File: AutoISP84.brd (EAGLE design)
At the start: 13 x 34.3 mm, 4 parts, among them J1 MCU, J2 BOARD, U1 ATTINY84-20PU, U2 ATTINY84-20PU

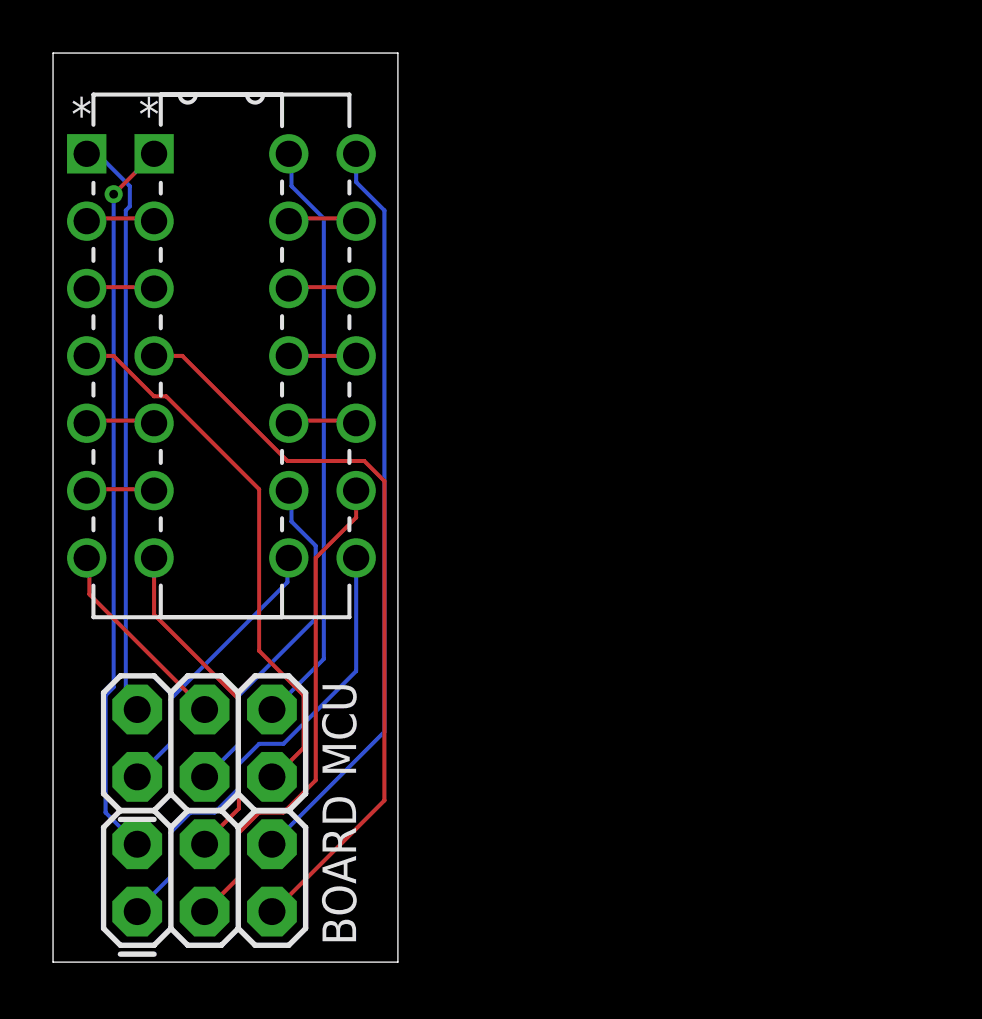
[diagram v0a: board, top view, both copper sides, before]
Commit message: Revise boards for better labelling and sane orientation, add AutoISP328
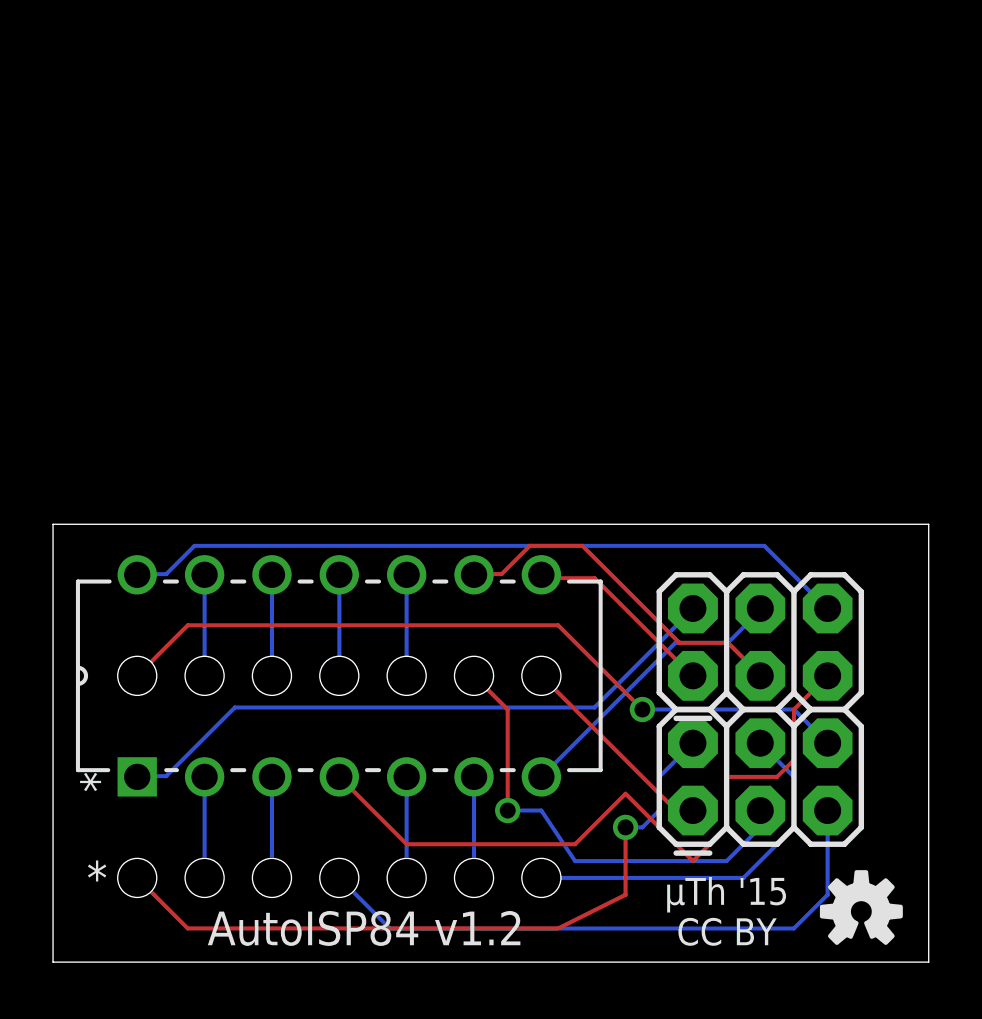
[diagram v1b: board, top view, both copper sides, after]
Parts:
- removed U2: ATTINY84-20PU, Atmel_By_element14_Batch_1-00:DIP254P762X533-14
- added JP1, JP2: (no value), SparkFun-Connectors:1X07_HOLES_ONLY
- added U$1: (no value), SparkFun-Aesthetics:OSHW-LOGO-S
- moved J1 21.3 mm to (24.1, 10.8)
- moved J2 21.3 mm to (24.1, 5.71)
- moved U1 9.55 mm to (18.4, 14.6), turned to 90 degrees
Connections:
- removed net N$11: J2.1, U2.8
- removed net N$13: J2.3, U2.9
- removed net N$9: J2.4, U2.7
- new net N$19: J2.4, JP1.7
- new net N$22: J2.1, JP2.1
- new net N$23: J2.3, JP2.2
- net N$12: now also JP2.6; no longer U2.13
- net N$14: now also JP1.5; no longer U2.5
- net N$15: now also JP1.3; no longer U2.3
- net N$16: now also JP1.2; no longer U2.2
- net N$17: now also JP1.6; no longer U2.6
- net N$18: now also JP2.5; no longer U2.12
- net N$2: now also JP1.1; no longer U2.1
- net N$20: now also JP2.4; no longer U2.11
- net N$21: now also JP2.3; no longer U2.10
- net N$3: now also JP2.7; no longer U2.14
- net N$7: now also JP1.4; no longer U2.4
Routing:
- net N$13: track 18.8 -> 0.00 mm
- net N$11: track 17.8 -> 0.00 mm
- net N$23: track 0.00 -> 17.3 mm, vias 0 -> 1
- net N$19: track 0.00 -> 14.0 mm
- net N$9: track 12.6 -> 0.00 mm
- net N$22: track 0.00 -> 7.82 mm
- net N$5: track 20.7 -> 26.4 mm
- net N$7: track 28.7 -> 22.9 mm
- net N$4: track 22.4 -> 27.5 mm
- net N$8: track 7.62 -> 10.9 mm
- net N$10: track 10.7 -> 7.34 mm
- net N$1: track 22.1 -> 23.6 mm
- net N$20: track 2.54 -> 3.81 mm
- net N$17: track 2.60 -> 3.81 mm
- net N$18: track 2.60 -> 3.81 mm
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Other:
- board size 13 x 34.3 mm -> 33 x 16.5 mm
- board text added: "*"
- board text added: "AutoISP84 v1.2"
- board text added: "µTh '15 CC BY"
- board text removed: "AutoISP84 v1.0 (C) µTh 2014"
